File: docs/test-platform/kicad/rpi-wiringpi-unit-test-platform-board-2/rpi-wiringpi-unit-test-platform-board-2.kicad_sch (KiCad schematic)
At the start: 18 parts, among them J1 IN_PWR_SERVO, J2 IN_I2C_SPI, J3 IN_CS_SR, J4 Servo, M1 ADS1115_0x48, SW1 SW_DIP_x01, U1 74HC595, U2 MCP3008, U3 MCP4922, U4 MCP42010

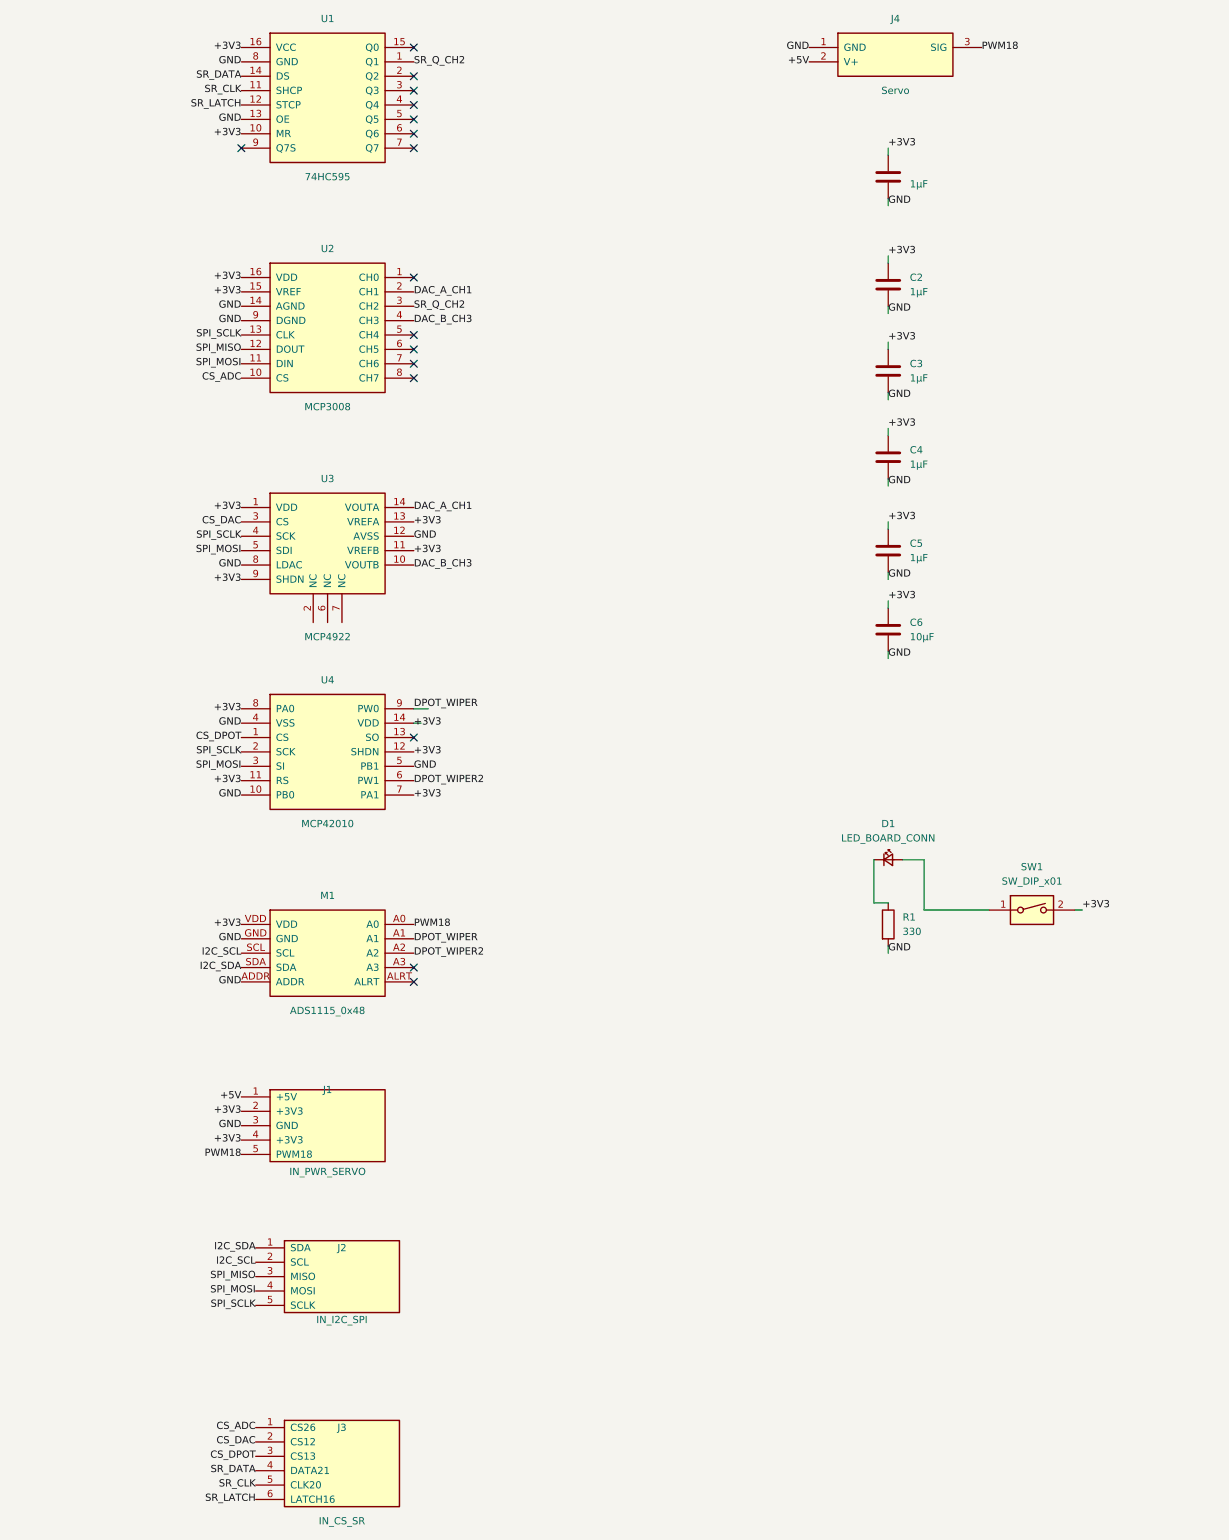
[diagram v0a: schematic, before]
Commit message: Updated boards
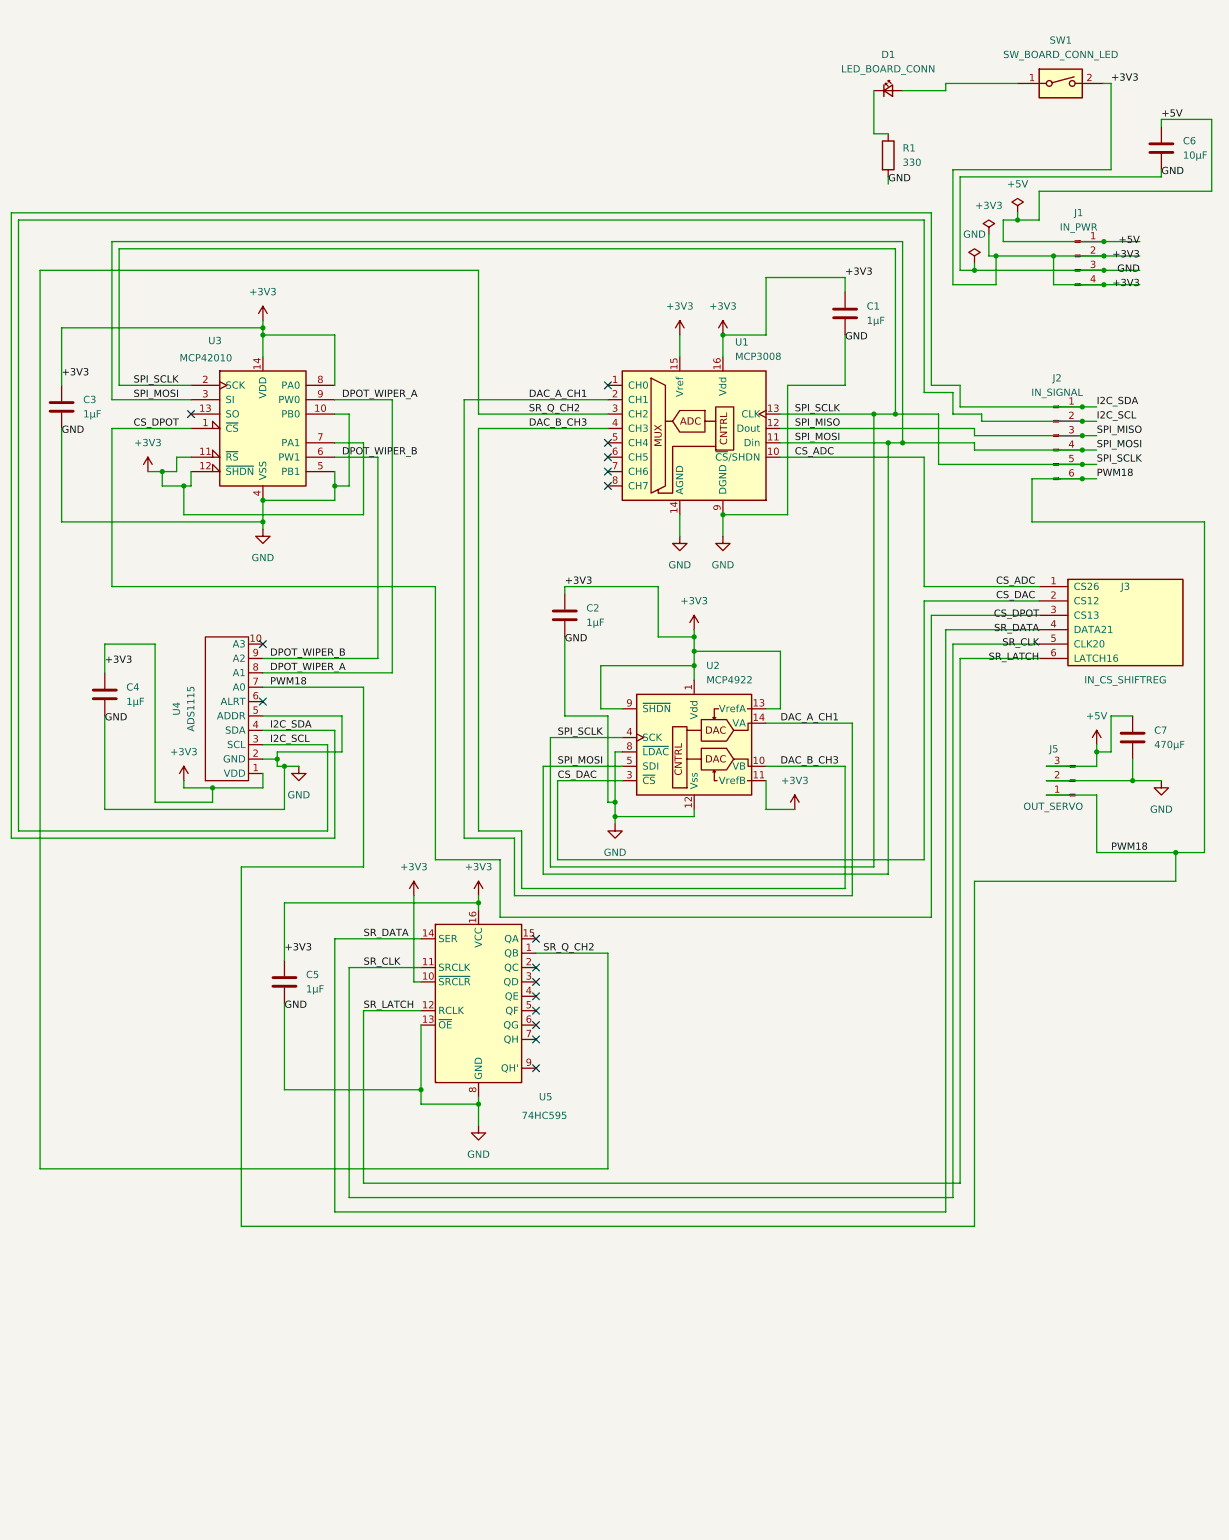
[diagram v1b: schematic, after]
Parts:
- removed J1: IN_PWR_SERVO, rpi-wiringpi-unit-test-platform-board-2:J1, symbol rpi-wiringpi-unit-test-platform-board-2:J1
- removed J2: IN_I2C_SPI, rpi-wiringpi-unit-test-platform-board-2:J2, symbol rpi-wiringpi-unit-test-platform-board-2:J2
- removed J4: Servo, rpi-wiringpi-unit-test-platform-board-2:J4, symbol rpi-wiringpi-unit-test-platform-board-2:J4
- removed M1: ADS1115_0x48, rpi-wiringpi-unit-test-platform-board-2:M1, symbol rpi-wiringpi-unit-test-platform-board-2:M1
- removed U1: 74HC595, rpi-wiringpi-unit-test-platform-board-2:U1, symbol rpi-wiringpi-unit-test-platform-board-2:U1
- removed U2: MCP3008, rpi-wiringpi-unit-test-platform-board-2:U2, symbol rpi-wiringpi-unit-test-platform-board-2:U2
- removed U3: MCP4922, rpi-wiringpi-unit-test-platform-board-2:U3, symbol rpi-wiringpi-unit-test-platform-board-2:U3
- removed U4: MCP42010, rpi-wiringpi-unit-test-platform-board-2:U4, symbol rpi-wiringpi-unit-test-platform-board-2:U4
- added C7: 470µF, Capacitor_THT:CP_Radial_D6.3mm_P2.50mm, symbol Device:C
- added J1: IN_PWR, Connector_JST:JST_XH_B4B-XH-A_1x04_P2.50mm_Vertical, symbol Connector:Conn_01x04_Pin
- added J2: IN_SIGNAL, Connector_JST:JST_XH_B6B-XH-A_1x06_P2.50mm_Vertical, symbol Connector:Conn_01x06_Pin
- added J5: OUT_SERVO, Connector_JST:JST_XH_B3B-XH-A_1x03_P2.50mm_Vertical, symbol Connector:Conn_01x03_Pin
- added U1: MCP3008, Package_DIP:DIP-16_W7.62mm, symbol Analog_ADC:MCP3008
- added U2: MCP4922, Package_DIP:DIP-14_W7.62mm, symbol Analog_DAC:MCP4922
- added U3: MCP42010, Package_DIP:DIP-14_W7.62mm, symbol Potentiometer_Digital:MCP42010
- added U4: ADS1115, RPi:ADS1115_Breakout, symbol RPi:ADS1115_ADC
- added U5: 74HC595, Package_DIP:DIP-16_W7.62mm, symbol 74xx:74HC595
- C6: footprint Capacitor_THT:C_Disc_D3.0mm_W2.0mm_P2.50mm -> Capacitor_THT:CP_Radial_D6.3mm_P2.50mm
- J3: value IN_CS_SR -> IN_CS_SHIFTREG; footprint rpi-wiringpi-unit-test-platform-board-2:J3 -> Connector_JST:JST_XH_B6B-XH-A_1x06_P2.50mm_Vertical
- SW1: value SW_DIP_x01 -> SW_BOARD_CONN_LED
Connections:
- net +3V3: now also J1.2 (Pin_2), J1.4 (Pin_4), U1.15 (Vref), U1.16 (Vdd), U2.1 (Vdd), U2.11 (VrefB), U2.13 (VrefA), U2.9 (~{SHDN}), U3.11 (~{RS}), U3.12 (~{SHDN}), U3.14 (VDD), U3.7 (PA1), U3.8 (PA0), U4.1 (VDD), U5.10 (~{SRCLR}), U5.16 (VCC); no longer C6.1
- net +5V: now also C6.1, C7.1, J1.1 (Pin_1), J5.3 (Pin_3)
- net CS_ADC: now also U1.10 (~{CS}/SHDN)
- net CS_DAC: now also U2.3 (~{CS})
- net CS_DPOT: now also U3.1 (~{CS})
- net DAC_A_CH1: now also U1.2 (CH1), U2.14 (VA)
- net DAC_B_CH3: now also U1.4 (CH3), U2.10 (VB)
- net GND: now also C7.2, J1.3 (Pin_3), J5.2 (Pin_2), U1.14 (AGND), U1.9 (DGND), U2.12 (Vss), U2.8 (~{LDAC}), U3.10 (PB0), U3.4 (VSS), U3.5 (PB1), U4.2 (GND), U4.5 (ADDR), U5.13 (~{OE}), U5.8 (GND)
- net I2C_SCL: now also J2.2 (Pin_2), U4.3 (SCL)
- net I2C_SDA: now also J2.1 (Pin_1), U4.4 (SDA)
- net PWM18: now also J2.6 (Pin_6), J5.1 (Pin_1), U4.7 (A0)
- net SPI_MISO: now also J2.3 (Pin_3), U1.12 (Dout)
- net SPI_MOSI: now also J2.4 (Pin_4), U1.11 (Din), U2.5 (SDI), U3.3 (SI)
- net SPI_SCLK: now also J2.5 (Pin_5), U1.13 (CLK), U2.4 (SCK), U3.2 (SCK)
- net SR_CLK: now also U5.11 (SRCLK)
- net SR_DATA: now also U5.14 (SER)
- net SR_LATCH: now also U5.12 (RCLK)
- net SR_Q_CH2: now also U1.3 (CH2), U5.1 (QB)
- new net DPOT_WIPER_A: U3.9 (PW0), U4.8 (A1)
- new net DPOT_WIPER_B: U3.6 (PW1), U4.9 (A2)
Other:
- moved on the sheet: C2, C3, C4, C5, C6, D1, J3, R1, SW1
